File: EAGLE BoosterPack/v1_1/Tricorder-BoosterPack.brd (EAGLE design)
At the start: 63.8 x 52.8 mm, 40 parts, among them U1 MAG3110, U2 LMT70LMT70, U3 HDC1000, U4 OPT3001, U5 LMP91000, U6 PGA900, U7 MICROSD

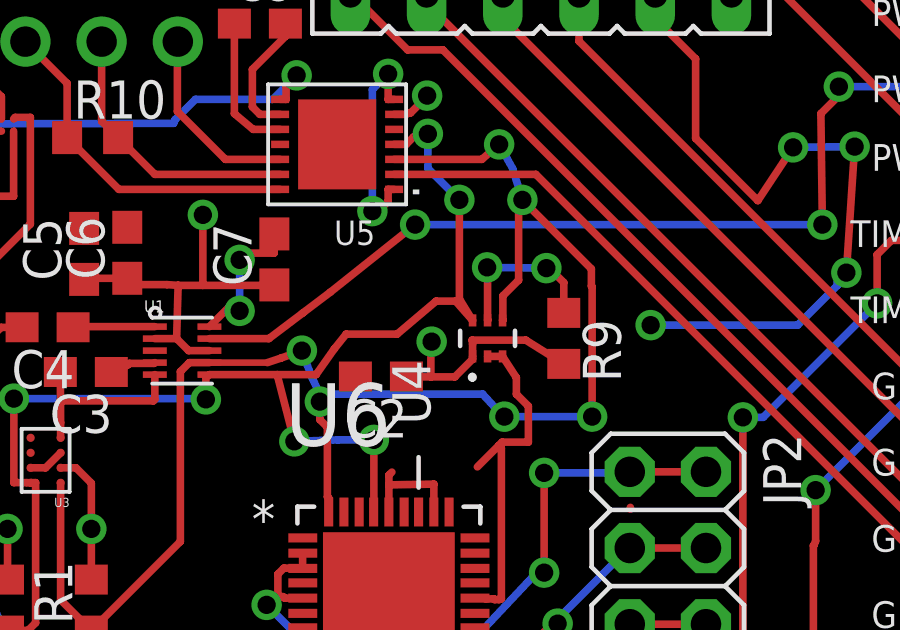
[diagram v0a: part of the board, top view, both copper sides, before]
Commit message: revised brd and sch
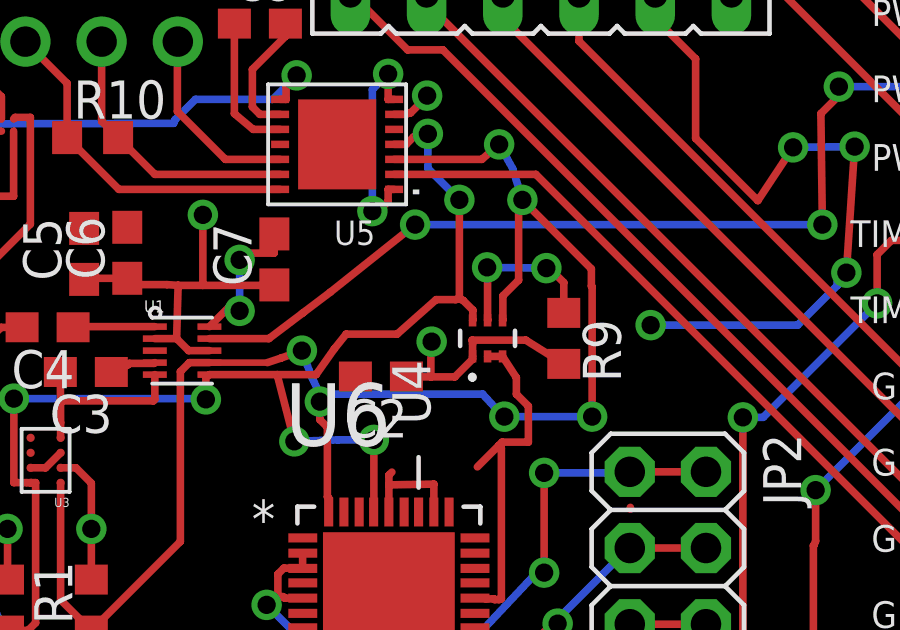
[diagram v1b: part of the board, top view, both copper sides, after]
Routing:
- net SDA: track 52.5 -> 51.9 mm
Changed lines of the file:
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@@
 <wire x1="39.225" y1="32.175" x2="39.225" y2="32.75" width="0.254" layer="1"/>
 <wire x1="39.225" y1="32.75" x2="36.925" y2="35.05" width="0.254" layer="1"/>
-<contactref element="U4" pad="4"/>
 <wire x1="36.8" y1="35" x2="36.925" y2="35.05" width="0.254" layer="1"/>
-<wire x1="36.275" y1="31.05" x2="36.265" y2="31.033" width="0.254" layer="1"/>
 <wire x1="36.8" y1="35" x2="36.8" y2="32.375" width="0.254" layer="1"/>
 <wire x1="36.8" y1="32.375" x2="36.275" y2="31.85" width="0.254" layer="1"/>
-<wire x1="36.275" y1="31.85" x2="36.275" y2="31.043" width="0.254" layer="1"/>
-<wire x1="36.275" y1="31.043" x2="36.265" y2="31.033" width="0.254" layer="1"/>
+<contactref element="U4" pad="4"/>
+<wire x1="36.275" y1="31.05" x2="36.275" y2="31.85" width="0.254" layer="1"/>
+<wire x1="36.275" y1="31.05" x2="36.265" y2="31.033" width="0.254" layer="1"/>
 </signal>
 <signal name="SDA">
@@
 <contactref element="U3" pad="A2"/>
 <contactref element="U1" pad="6"/>
-<contactref element="U4" pad="6"/>
 <wire x1="20.7" y1="25.625" x2="20.55" y2="25.625" width="0.254" layer="1"/>
 <wire x1="20.7" y1="20.95" x2="20.7" y2="25.625" width="0.254" layer="1"/>
@@
 <wire x1="34.825" y1="35.05" x2="33.775" y2="36.1" width="0.254" layer="16"/>
 <wire x1="34.825" y1="31.75" x2="34.825" y2="35.05" width="0.254" layer="1"/>
-<wire x1="34.825" y1="31.75" x2="35.265" y2="31.033" width="0.254" layer="1"/>
 <via x="33.775" y="37.25" extent="1-16" drill="0.6096"/>
 <via x="34.825" y="35.05" extent="1-16" drill="0.6096"/>
@@
 <wire x1="31.05" y1="30.575" x2="30.65" y2="30.075" width="0.254" layer="1"/>
 <wire x1="32.75" y1="30.575" x2="31.05" y2="30.575" width="0.254" layer="1"/>
-<wire x1="34.05" y1="31.675" x2="32.75" y2="30.575" width="0.254" layer="1"/>
-<wire x1="34.7" y1="31.675" x2="34.05" y2="31.675" width="0.254" layer="1"/>
-<wire x1="34.7" y1="31.675" x2="35.265" y2="31.033" width="0.254" layer="1"/>
+<wire x1="34.05" y1="31.725" x2="32.75" y2="30.575" width="0.254" layer="1"/>
 <contactref element="U6" pad="33"/>
+<wire x1="34.7" y1="31.725" x2="34.05" y2="31.725" width="0.254" layer="1"/>
 <wire x1="31.975" y1="27.05" x2="31.975" y2="24.65" width="0.254" layer="1"/>
 <wire x1="30.775" y1="27.05" x2="31.975" y2="27.05" width="0.254" layer="16"/>
@@
 <via x="31.975" y="27.05" extent="1-16" drill="0.6096"/>
 <via x="29.325" y="27" extent="1-16" drill="0.6096"/>
+<contactref element="U4" pad="6"/>
+<wire x1="35.275" y1="31.375" x2="34.95" y2="31.7" width="0.254" layer="1"/>
+<wire x1="35.275" y1="31.05" x2="35.275" y2="31.375" width="0.254" layer="1"/>
+<wire x1="34.95" y1="31.7" x2="34.825" y2="31.75" width="0.254" layer="1"/>
+<wire x1="35.275" y1="31.05" x2="35.265" y2="31.033" width="0.254" layer="1"/>
+<wire x1="34.7" y1="31.725" x2="34.825" y2="31.75" width="0.254" layer="1"/>
 </signal>
 <signal name="N$5">
